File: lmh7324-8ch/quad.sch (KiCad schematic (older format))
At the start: 37 parts, among them IC201 lmh7324

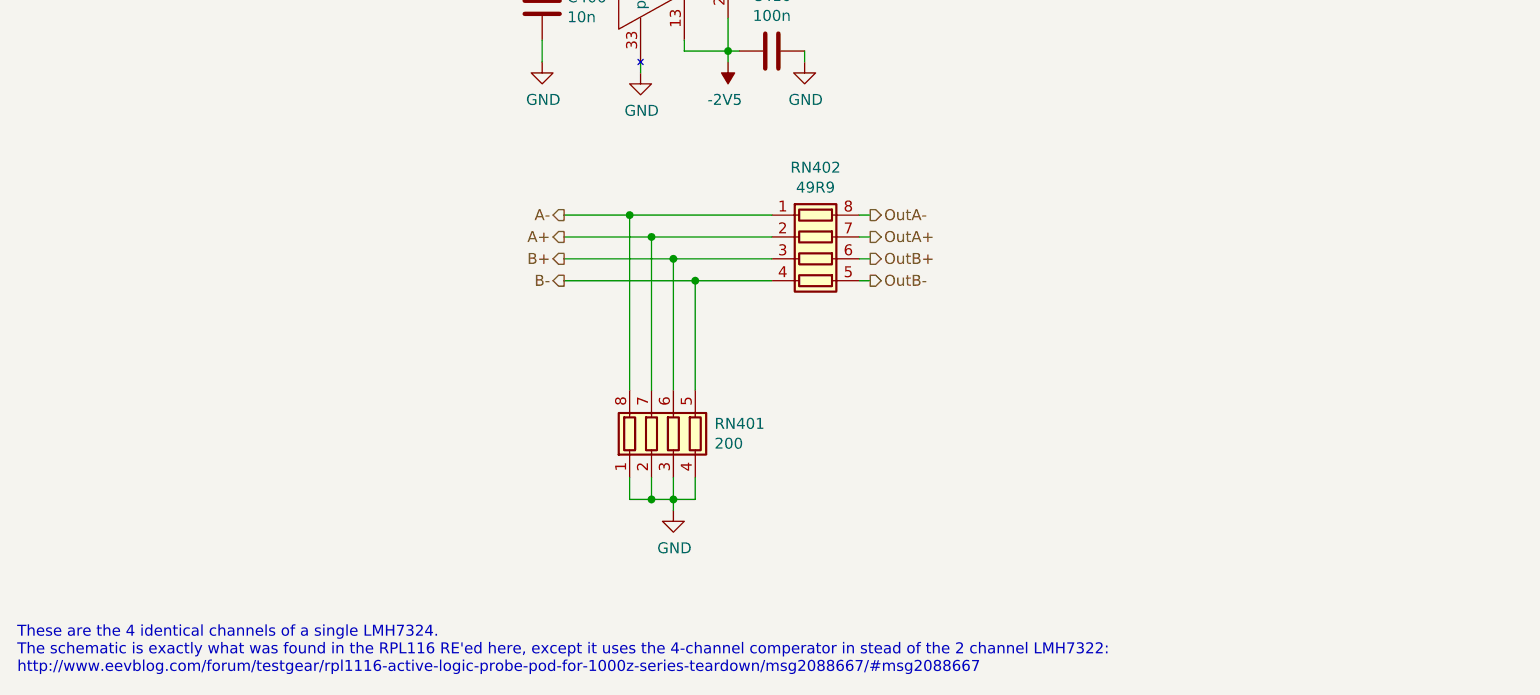
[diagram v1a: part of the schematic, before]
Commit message: Added proper readme
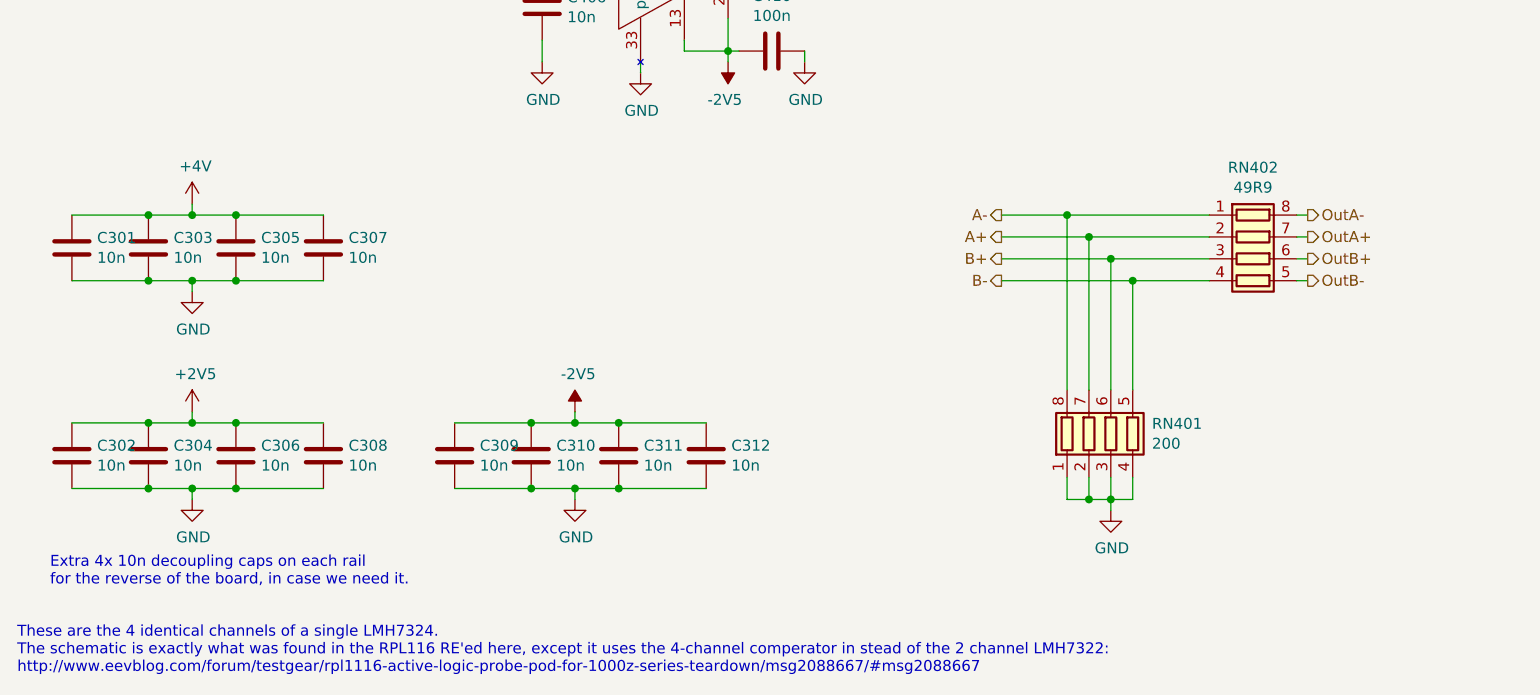
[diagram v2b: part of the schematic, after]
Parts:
- added C301, C302, C303, C304, C305, C306, C307, C308, C309, C310, C311, C312: 10n, Capacitor_SMD:C_0402_1005Metric, symbol Device:C
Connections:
- net +2V5: now also C302.1, C304.1, C306.1, C308.1
- net +4V: now also C301.1, C303.1, C305.1, C307.1
- net -2V5: now also C309.1, C310.1, C311.1, C312.1
- net GND: now also C301.2, C302.2, C303.2, C304.2, C305.2, C306.2, C307.2, C308.2, C309.2, C310.2, C311.2, C312.2
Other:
- note added: "Extra 4x 10n decoupling caps on each rail\nfor the reverse of the board, in case we need it."
- moved on the sheet: RN401, RN402
